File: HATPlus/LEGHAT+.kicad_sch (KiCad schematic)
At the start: 25 parts, among them J1 Conn_02x20_Odd_Even, J2 Conn_01x02, J3 Conn_01x08, Q2 CSD18540Q5B, SW1 SW_Push, U4 LTC4373IDD-PBF

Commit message: newnewenew
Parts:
- J1: footprint SSM-120-F-DV:SAMTEC_SSM-120-X-DV -> Connector_PinSocket_2.54mm:PinSocket_2x20_P2.54mm_Vertical
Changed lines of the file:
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@@
 			)
 		)
-		(property "Footprint" "SSM-120-F-DV:SAMTEC_SSM-120-X-DV"
+		(property "Footprint" "Connector_PinSocket_2.54mm:PinSocket_2x20_P2.54mm_Vertical"
 			(at 248.92 81.28 0)
 			(hide yes)

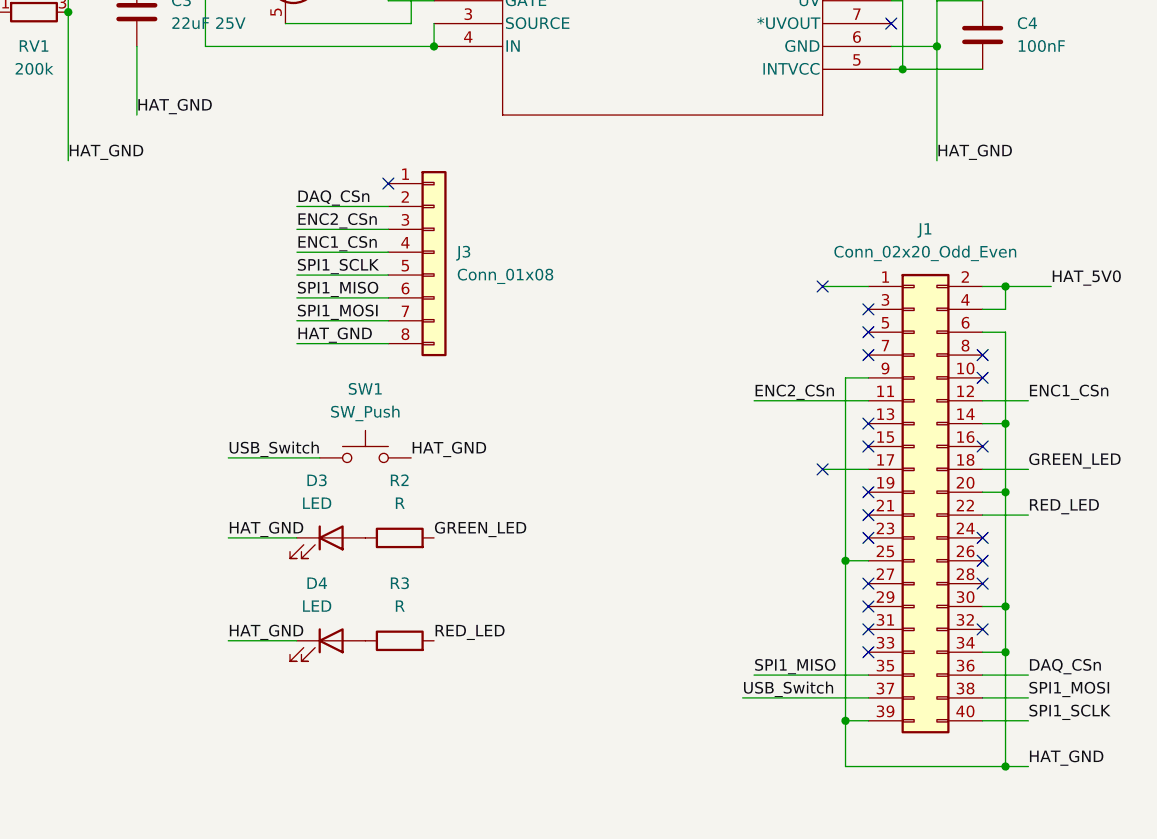
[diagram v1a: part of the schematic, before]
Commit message: nununununu
nunununu
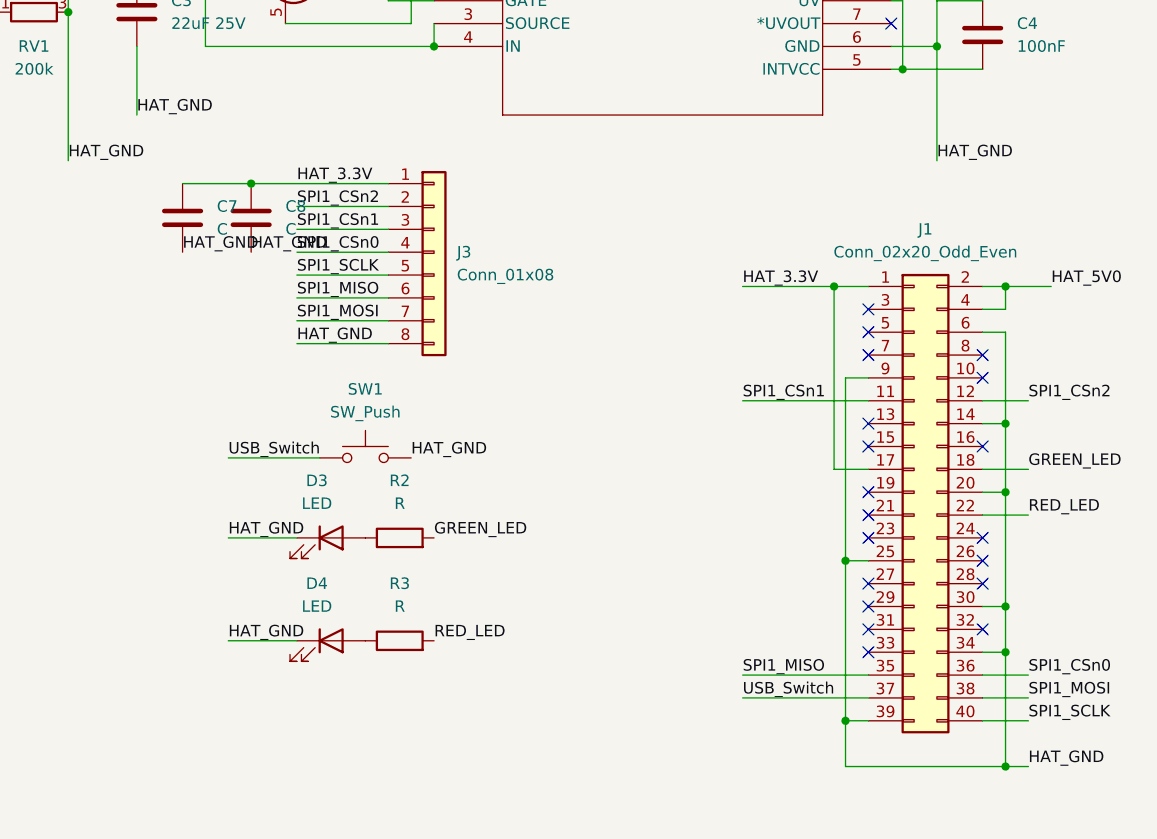
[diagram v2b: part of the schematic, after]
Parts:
- added C7, C8: C, Capacitor_SMD:C_0603_1608Metric, symbol Device:C
- D1: footprint (none) -> Package_TO_SOT_SMD:TO-277A
- J3: footprint Connector_JST:JST_GH_BM08B-GHS-TBT_1x08-1MP_P1.25mm_Vertical -> Connector_Molex:Molex_MicroClasp_55932-0810_1x08_P2.00mm_Vertical
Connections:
- net HAT_GND: now also C7.2, C8.2
- net HAT_3.3V: now reaches J1.1 (Pin_1)
- net HAT_3.3V: now also J1.17 (Pin_17), J3.1 (Pin_1), C7.1, C8.1
- net DAQ_CSn renamed SPI1_CSn0
- net SPI1_CSn0: now also J3.4 (Pin_4); no longer J3.2 (Pin_2)
- net ENC1_CSn renamed SPI1_CSn2
- net SPI1_CSn2: now also J3.2 (Pin_2); no longer J3.4 (Pin_4)
- net ENC2_CSn renamed SPI1_CSn1
- no-connect marks 24 -> 21

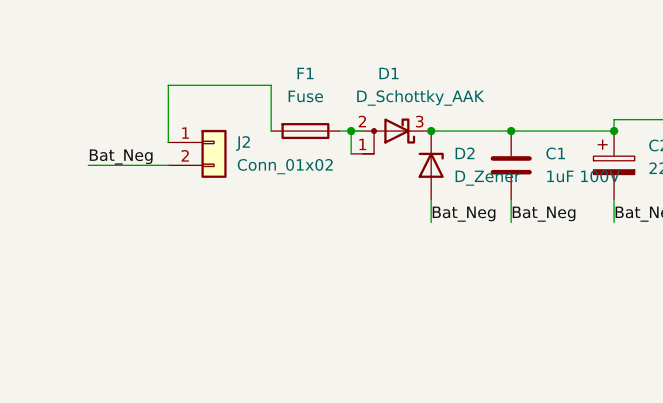
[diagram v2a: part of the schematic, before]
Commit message: almost final
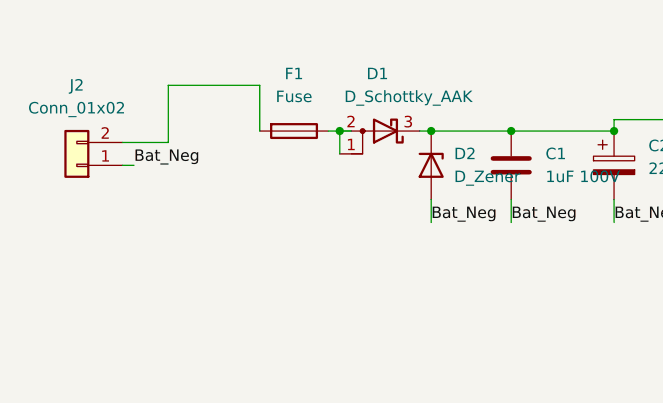
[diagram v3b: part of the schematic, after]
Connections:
- net Bat_Neg: now also J2.1 (Pin_1); no longer J2.2 (Pin_2)
- net at F1.2: now also J2.2 (Pin_2); no longer J2.1 (Pin_1)
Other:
- moved on the sheet: D1, F1, J2
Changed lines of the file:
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@@
 	)
 	(junction
-		(at 44.45 24.13)
+		(at 43.18 24.13)
 		(diameter 0)
 		(color 0 0 0 0)
@@
 	(wire
 		(pts
-			(xy 35.56 24.13) (xy 35.56 19.05)
-		)
-		(stroke
-			(width 0)
-			(type default)
-		)
-	)
-	(wire
-		(pts
 			(xy 170.18 19.05) (xy 170.18 22.86)
 		)
@@
 	(wire
 		(pts
-			(xy 15.24 27.94) (xy 24.13 27.94)
+			(xy 20.32 27.94) (xy 19.05 27.94)
 		)
 		(stroke
@@
 	(wire
 		(pts
+			(xy 34.29 19.05) (xy 34.29 24.13)
+		)
+		(stroke
+			(width 0)
+			(type default)
+		)
+	)
+	(wire
+		(pts
 			(xy 240.03 78.74) (xy 240.03 58.42)
 		)
@@
 	(wire
 		(pts
-			(xy 44.45 24.13) (xy 43.18 24.13)
+			(xy 43.18 24.13) (xy 41.91 24.13)
 		)
 		(stroke
@@
 	(wire
 		(pts
-			(xy 44.45 24.13) (xy 44.45 26.67)
+			(xy 43.18 24.13) (xy 43.18 26.67)
 		)
 		(stroke
@@
 	(wire
 		(pts
+			(xy 52.07 24.13) (xy 53.34 24.13)
+		)
+		(stroke
+			(width 0)
+			(type default)
+		)
+	)
+	(wire
+		(pts
 			(xy 195.58 29.21) (xy 195.58 31.75)
 		)
@@
 	(wire
 		(pts
-			(xy 44.45 24.13) (xy 45.72 24.13)
+			(xy 43.18 24.13) (xy 44.45 24.13)
 		)
 		(stroke
@@
 	(wire
 		(pts
-			(xy 24.13 19.05) (xy 35.56 19.05)
+			(xy 24.13 19.05) (xy 34.29 19.05)
 		)
 		(stroke
@@
 	(wire
 		(pts
+			(xy 19.05 25.4) (xy 24.13 25.4)
+		)
+		(stroke
+			(width 0)
+			(type default)
+		)
+	)
+	(wire
+		(pts
 			(xy 193.04 24.13) (xy 195.58 24.13)
 		)
@@
 	)
 	(label "Bat_Neg"
-		(at 15.24 27.94 0)
+		(at 20.32 27.94 0)
 		(effects
 			(font
@@
 	(symbol
 		(lib_id "Connector_Generic:Conn_01x02")
-		(at 29.21 25.4 0)
+		(at 13.97 27.94 180)
 		(unit 1)
 		(body_style 1)
@@
 		(fields_autoplaced yes)
 		(property "Reference" "J2"
-			(at 31.75 25.3999 0)
+			(at 13.97 19.05 0)
 			(show_name no)
 			(do_not_autoplace no)
@@
 					(size 1.27 1.27)
 				)
-				(justify left)
 			)
 		)
 		(property "Value" "Conn_01x02"
-			(at 31.75 27.9399 0)
+			(at 13.97 21.59 0)
 			(show_name no)
 			(do_not_autoplace no)
@@
 					(size 1.27 1.27)
 				)
-				(justify left)
 			)
 		)
 		(property "Footprint" "Connector_AMASS:AMASS_XT30UPB-F_1x02_P5.0mm_Vertical"
-			(at 29.21 25.4 0)
+			(at 13.97 27.94 0)
 			(hide yes)
 			(show_name no)
@@
 		)
 		(property "Datasheet" ""
-			(at 29.21 25.4 0)
+			(at 13.97 27.94 0)
 			(hide yes)
 			(show_name no)
@@
 		)
 		(property "Description" "Generic connector, single row, 01x02, script generated (kicad-library-utils/schlib/autogen/connector/)"
-			(at 29.21 25.4 0)
+			(at 13.97 27.94 0)
 			(hide yes)
 			(show_name no)
@@
 	(symbol
 		(lib_id "Device:Fuse")
-		(at 39.37 24.13 270)
+		(at 38.1 24.13 270)
 		(unit 1)
 		(body_style 1)
@@
 		(fields_autoplaced yes)
 		(property "Reference" "F1"
-			(at 39.37 17.78 90)
+			(at 38.1 17.78 90)
 			(show_name no)
 			(do_not_autoplace no)
@@
 		)
 		(property "Value" "Fuse"
-			(at 39.37 20.32 90)
+			(at 38.1 20.32 90)
 			(show_name no)
 			(do_not_autoplace no)
@@
 		)
 		(property "Footprint" "belfuse0680L3000-05:FUSC6125X279N"
-			(at 39.37 22.352 90)
+			(at 38.1 22.352 90)
 			(hide yes)
 			(show_name no)
@@
 		)
 		(property "Datasheet" ""
-			(at 39.37 24.13 0)
+			(at 38.1 24.13 0)
 			(hide yes)
 			(show_name no)
@@
 		)
 		(property "Description" "Fuse"
-			(at 39.37 24.13 0)
+			(at 38.1 24.13 0)
 			(hide yes)
 			(show_name no)
@@
 	(symbol
 		(lib_id "Device:D_Schottky_AAK")
-		(at 49.53 24.13 180)
+		(at 48.26 24.13 180)
 		(unit 1)
 		(body_style 1)
@@
 		(dnp no)
 		(property "Reference" "D1"
-			(at 48.641 17.78 0)
+			(at 47.371 17.78 0)
 			(show_name no)
 			(do_not_autoplace no)
@@
 		)
 		(property "Value" "D_Schottky_AAK"
-			(at 52.07 20.32 0)
+			(at 50.8 20.32 0)
 			(show_name no)
 			(do_not_autoplace no)
@@
 		)
 		(property "Footprint" "Package_TO_SOT_SMD:TO-277A"
-			(at 49.53 24.13 0)
+			(at 48.26 24.13 0)
 			(hide yes)
 			(show_name no)
@@
 		)
 		(property "Datasheet" ""
-			(at 49.53 24.13 0)
+			(at 48.26 24.13 0)
 			(hide yes)
 			(show_name no)
@@
 		)
 		(property "Description" "Schottky diode, anode on pins 1 and 2"
-			(at 49.53 24.13 0)
+			(at 48.26 24.13 0)
 			(hide yes)
 			(show_name no)
